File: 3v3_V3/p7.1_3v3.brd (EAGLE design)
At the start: 27.8 x 61.8 mm, 17 parts, among them Q1 SSM3J3228R, Q2 SSM3J3228R, U2 DS3231ST&R

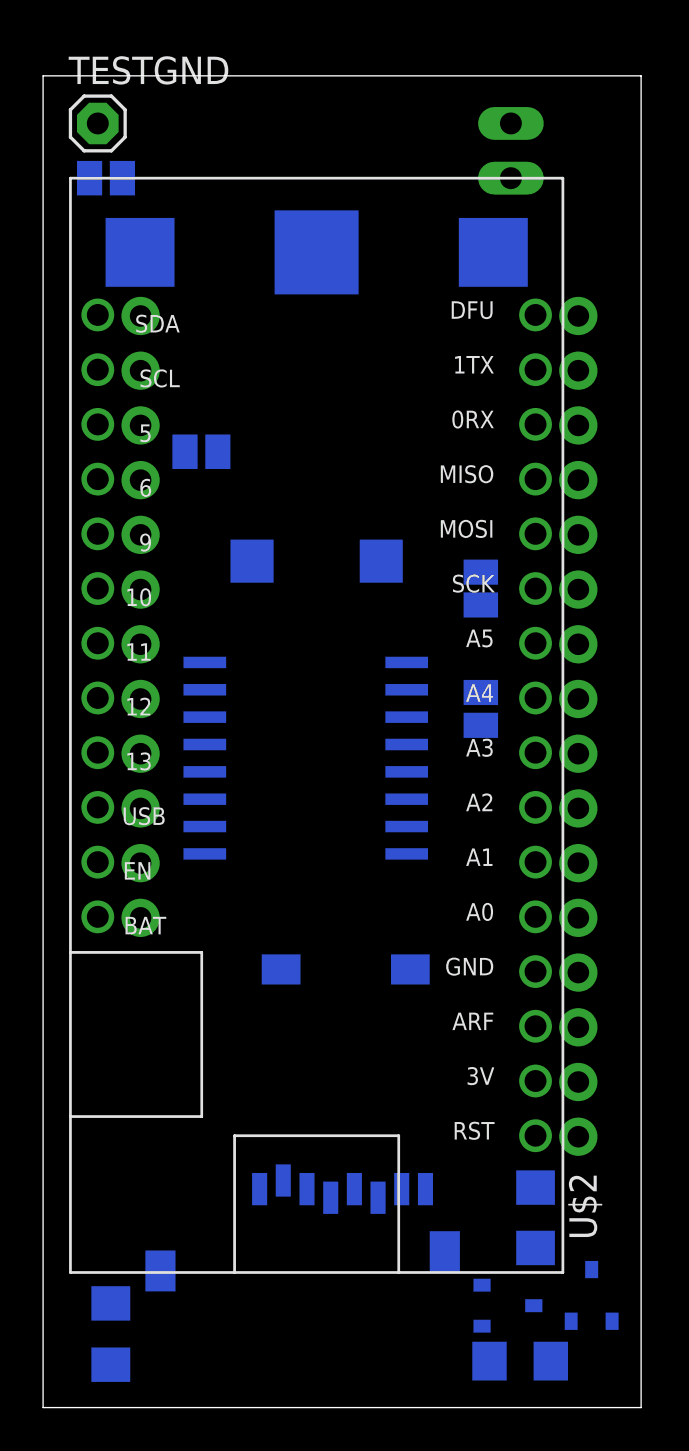
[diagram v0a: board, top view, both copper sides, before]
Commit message: Add files via upload
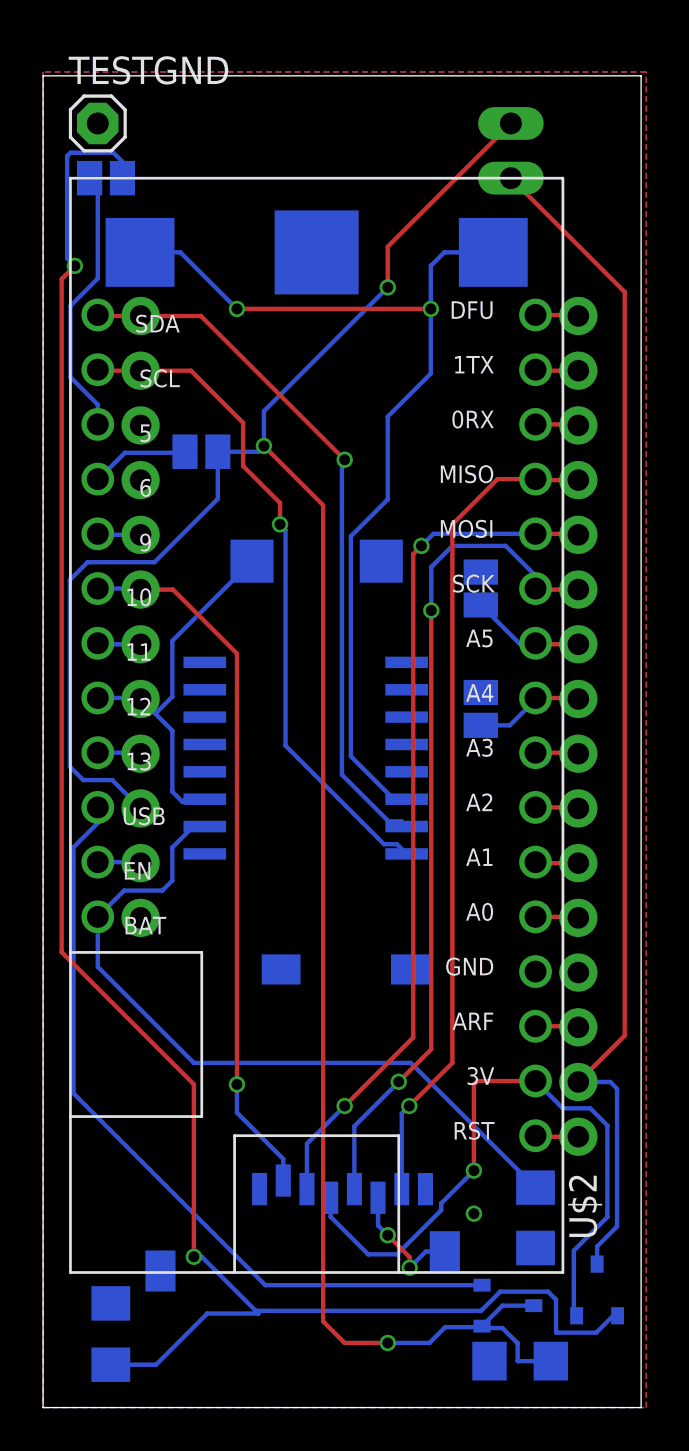
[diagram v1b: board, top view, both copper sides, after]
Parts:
- moved Q2 0.36 mm to (25.7, 0.46)
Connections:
- removed net 3V: MS1.2
- new net 0RX: MS1.14, U$2.0RX
- new net 11: MS1.23, U$2.11
- new net 13: MS1.25, U$2.13
- new net 1TX: MS1.15, U$2.1TX
- new net 9: MS1.21, U$2.9
- new net A0: MS1.5, U$2.A0
- new net A1: MS1.6, U$2.A1
- new net A2: MS1.7, U$2.A2
- new net A3: MS1.8, U$2.A3
- new net ARF: MS1.3, U$2.ARF
- new net DFU: MS1.16, U$2.DFU
- new net EN: MS1.27, U$2.EN
- new net N$7: MS1.20
- new net N$8: MS1.19
- new net RESET: MS1.1, U$2.RST
- net 3VRAIL: now also EXT|RTC_INT.1, MS1.2
- net 5VRAIL: now also EXT|RTC_INT.2, MS1.26
- net RTC_INT: no longer EXT|RTC_INT.2
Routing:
- net 5VRAIL: track 0.00 -> 102.4 mm, vias 0 -> 3
- net OUTPUT3V3: track 0.00 -> 88.7 mm, vias 0 -> 2
- net 3VRAIL: track 0.00 -> 55.5 mm
- net N$2: track 0.00 -> 45.5 mm, vias 0 -> 2
- net DI: track 0.00 -> 39.6 mm, vias 0 -> 2
- net CLK: track 0.00 -> 38.8 mm, vias 0 -> 2
- net DO: track 0.00 -> 38.6 mm, vias 0 -> 1
- net 5VUSB: track 0.00 -> 36.4 mm
- net VBATT: track 0.00 -> 34.5 mm
- net CS: track 0.00 -> 33.1 mm, vias 0 -> 1
- net SDA: track 0.00 -> 32.9 mm, vias 0 -> 1
- net SCL: track 0.00 -> 31.3 mm, vias 0 -> 1
- net +3V3: track 0.00 -> 30.7 mm, vias 0 -> 1
- net RTC_INT: track 0.00 -> 17.6 mm
- net N$3: track 0.00 -> 12.6 mm
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- added copper zone on layer 1, net GND
- added copper zone on layer 16, net GND
